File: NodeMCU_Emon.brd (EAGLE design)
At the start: 67.6 x 44.8 mm, 20 parts, among them IC1-D24V5F5 7805T, J3 10p-2.54, J6 ST-PJ-312, J7 H4P-SMD-2.0

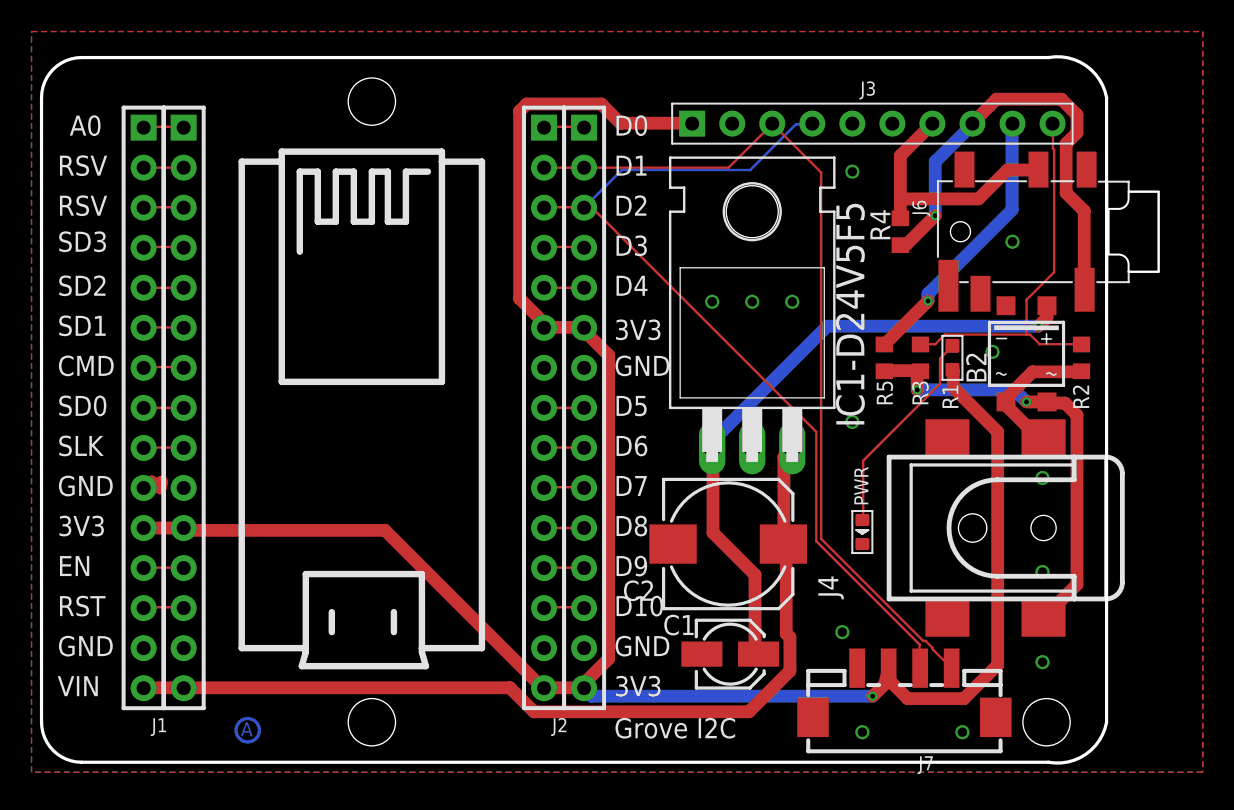
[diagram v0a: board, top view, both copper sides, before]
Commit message: Finished routing and fixups
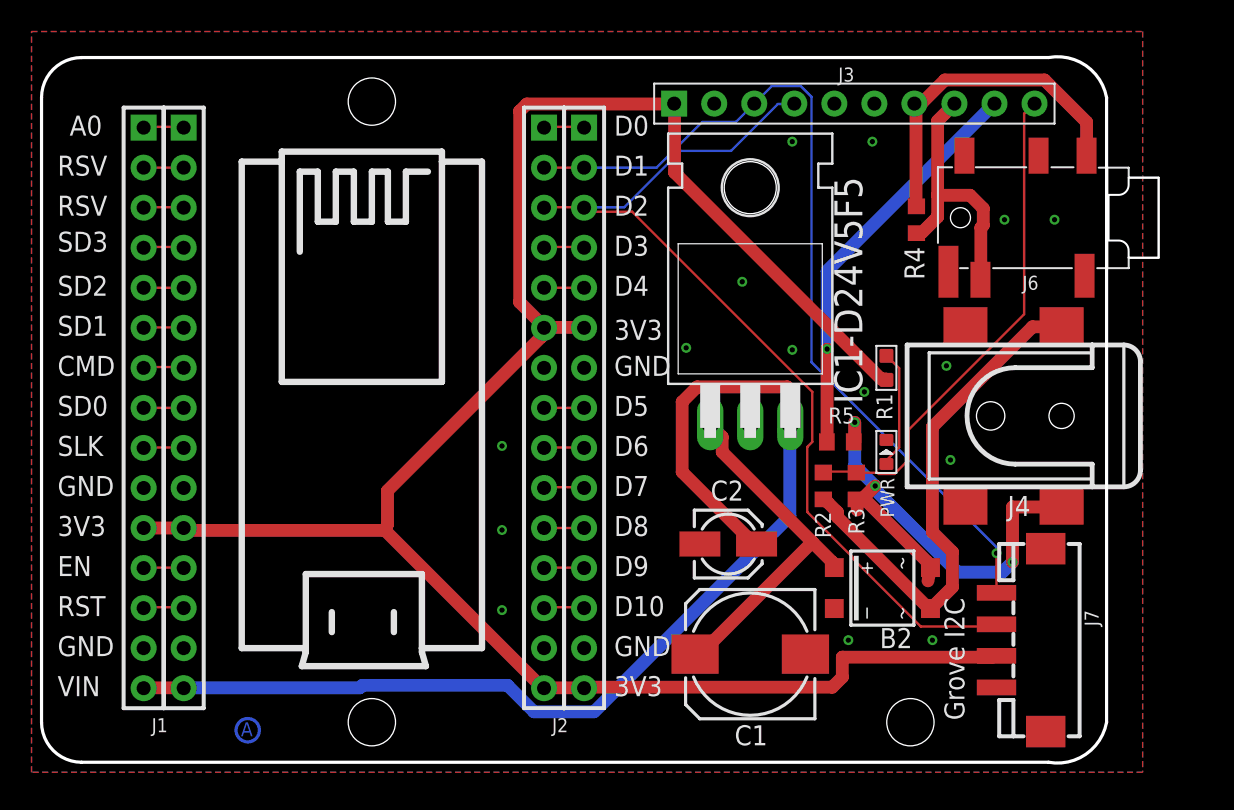
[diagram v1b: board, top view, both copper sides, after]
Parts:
- C1: value 10uF -> 100uF; device adafruit:153CLV-0405 -> adafruit:175TMP-0808
- C2: value 100uF -> 10uF; device adafruit:175TMP-0808 -> adafruit:153CLV-0405
- R4: value 330R -> 100R
- moved R2 18.3 mm to (49.6, 17.5)
- moved B2 17.4 mm to (53.3, 11.0), turned to 90 degrees
- moved R3 9.09 mm to (51.7, 17.5)
- moved J4 7.20 mm to (62.5, 22.0)
- moved J7 6.11 mm to (60.6, 7.75), turned to 270 degrees
- moved R5 6.02 mm to (50.7, 20.3), turned to 0 degrees
- moved PWR 5.30 mm to (53.6, 19.7), turned to 90 degrees
- moved R1 4.24 mm to (53.6, 25.0)
- moved J3 1.71 mm to (51.6, 41.8)
- moved IC1-D24V5F5 1.53 mm to (45.0, 31.6)
- moved R4 1.27 mm to (55.5, 34.4)
- moved C1 1.27 mm to (45.0, 6.86), turned to 180 degrees
- moved J6 0.89 mm to (70.9, 34.5)
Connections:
- net I_AC+: now also J6.COM1; no longer J6.R
- net I_AC-: now also J6.L; no longer J6.COM2
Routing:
- net N$3: track 9.16 -> 33.3 mm
- net N$4: track 40.0 -> 22.7 mm, vias 1 -> 0
- net VIN: track 57.3 -> 73.9 mm
- net I_AC-: track 29.4 -> 17.2 mm, vias 1 -> 0
- net A2: track 17.4 -> 25.9 mm
- net 3V3: track 134.4 -> 127.1 mm, vias 1 -> 0
- net V_AC+: track 24.9 -> 31.8 mm
- net N$1: track 13.4 -> 7.54 mm
- net V_AC-: track 28.1 -> 33.1 mm, vias 2 -> 3
- net I_AC+: track 16.4 -> 21.3 mm
- net D2: track 57.6 -> 61.1 mm
- net GND: track 2.11 -> 0.00 mm, vias 13 -> 15
- net D1: track 55.0 -> 55.7 mm, vias 0 -> 1
